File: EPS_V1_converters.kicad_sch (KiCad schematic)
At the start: 46 parts, among them U2 TPS62132RGTR, U3 TPS62133RGTR, U4 MP28167GQ-Z, U6 TPS61088RHLR

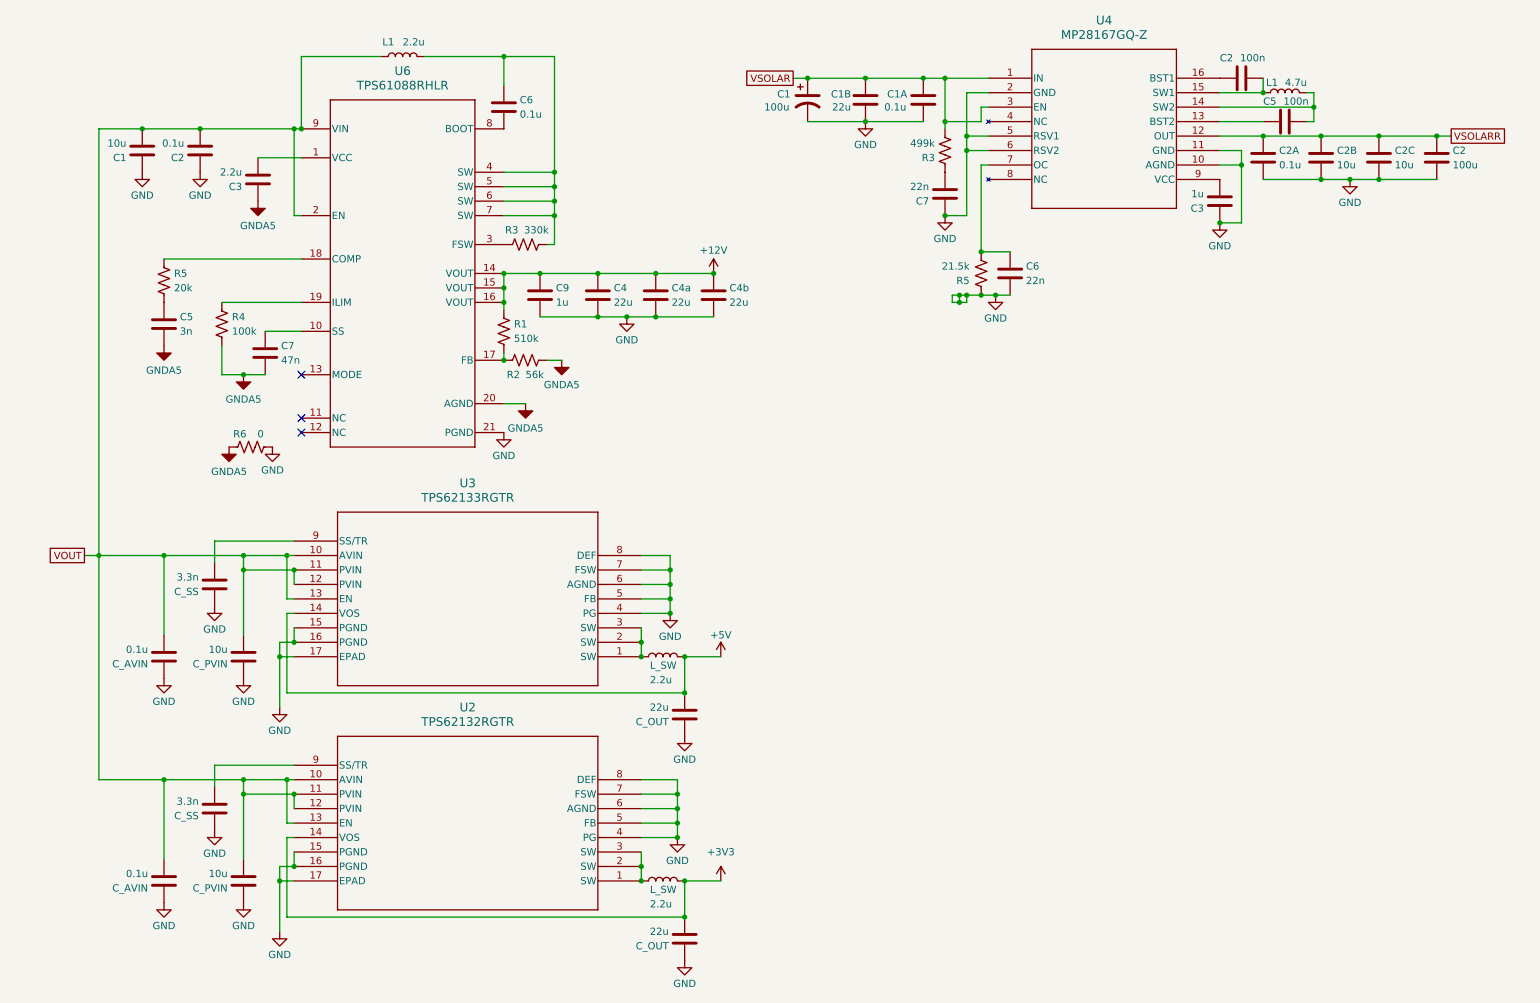
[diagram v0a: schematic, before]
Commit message: Clarify global net naming, other minor fixes
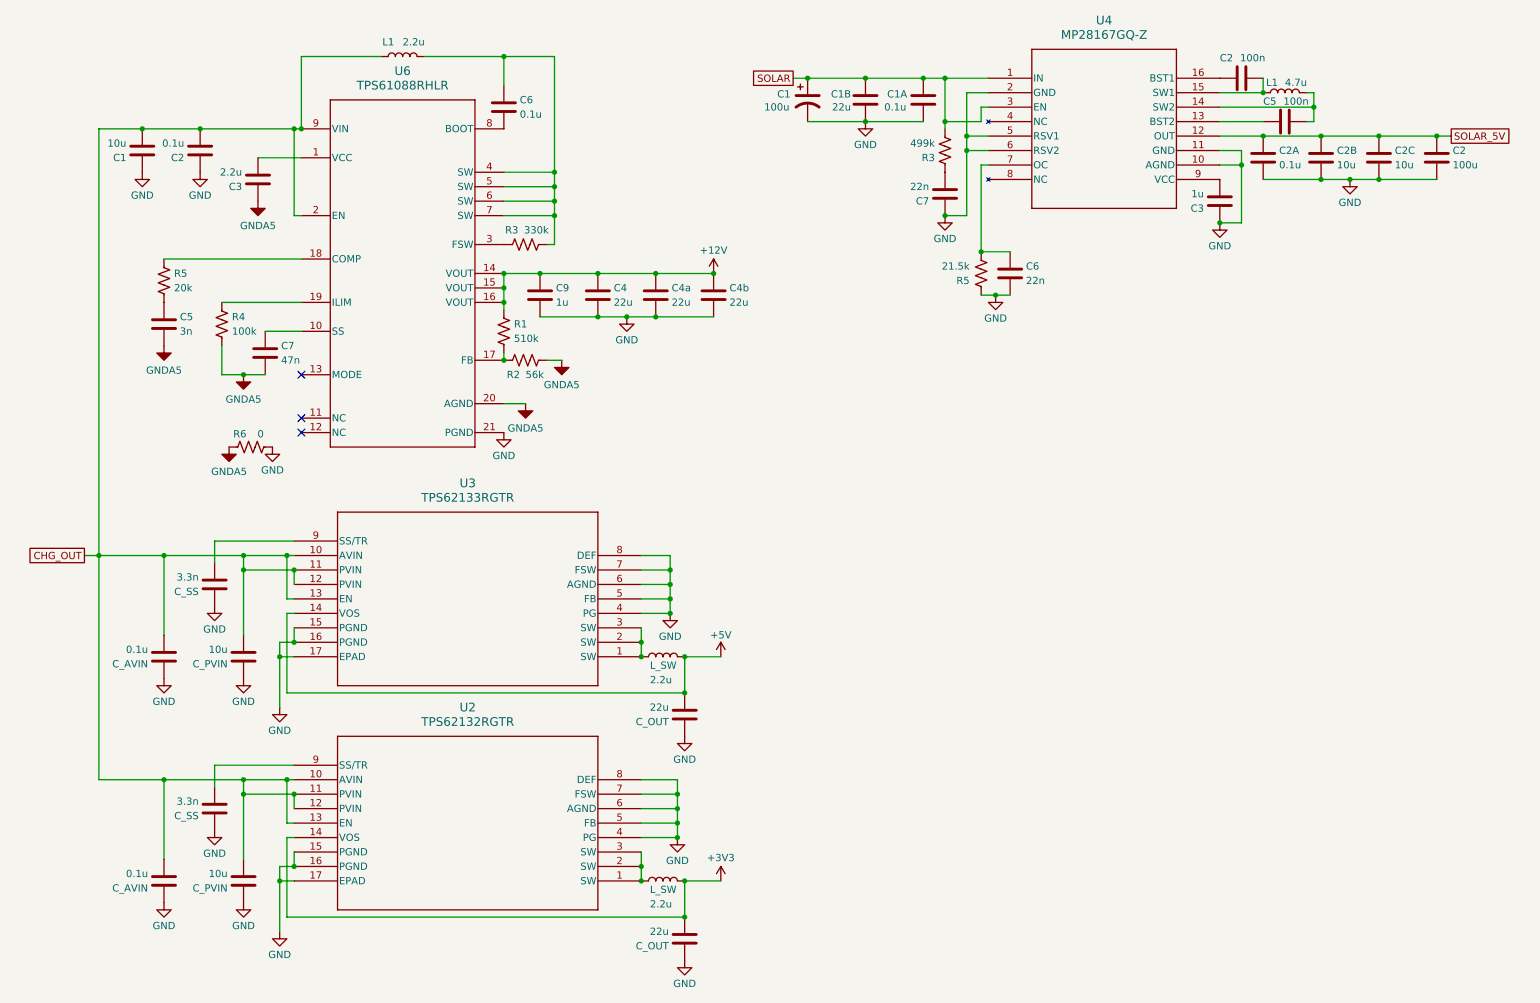
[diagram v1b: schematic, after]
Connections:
- net VOUT renamed CHG_OUT
- net VSOLAR renamed SOLAR
- net VSOLARR renamed SOLAR_5V
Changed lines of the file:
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@@
-	)
-	(junction
-		(at 186.69 68.58)
-		(diameter 0)
-		(color 0 0 0 0)
 	)
 	(junction
@@
 	)
 	(junction
-		(at 185.42 68.58)
-		(diameter 0)
-		(color 0 0 0 0)
-	)
-	(junction
 		(at 132.08 72.39)
 		(diameter 0)
@@
 	)
 	(junction
-		(at 189.23 68.58)
-		(diameter 0)
-		(color 0 0 0 0)
-	)
-	(junction
 		(at 114.3 49.53)
 		(diameter 0)
@@
 	(junction
 		(at 68.58 39.37)
-		(diameter 0)
-		(color 0 0 0 0)
-	)
-	(junction
-		(at 185.42 69.85)
 		(diameter 0)
 		(color 0 0 0 0)
@@
 	(wire
 		(pts
-			(xy 189.23 68.58) (xy 186.69 68.58)
-		)
-		(stroke
-			(width 0)
-			(type default)
-		)
-	)
-	(wire
-		(pts
 			(xy 114.3 59.69) (xy 113.03 59.69)
 		)
@@
 	(wire
 		(pts
-			(xy 186.69 68.58) (xy 186.69 69.85)
-		)
-		(stroke
-			(width 0)
-			(type default)
-		)
-	)
-	(wire
-		(pts
 			(xy 186.69 33.02) (xy 190.5 33.02)
 		)
@@
 	(wire
 		(pts
-			(xy 184.15 69.85) (xy 185.42 69.85)
-		)
-		(stroke
-			(width 0)
-			(type default)
-		)
-	)
-	(wire
-		(pts
 			(xy 190.5 35.56) (xy 189.23 35.56)
 		)
@@
 	(wire
 		(pts
-			(xy 185.42 68.58) (xy 185.42 69.85)
-		)
-		(stroke
-			(width 0)
-			(type default)
-		)
-	)
-	(wire
-		(pts
 			(xy 105.41 49.53) (xy 114.3 49.53)
 		)
@@
 	(wire
 		(pts
-			(xy 184.15 68.58) (xy 184.15 69.85)
-		)
-		(stroke
-			(width 0)
-			(type default)
-		)
-	)
-	(wire
-		(pts
 			(xy 105.41 46.99) (xy 114.3 46.99)
 		)
@@
 	(wire
 		(pts
-			(xy 185.42 68.58) (xy 184.15 68.58)
-		)
-		(stroke
-			(width 0)
-			(type default)
-		)
-	)
-	(wire
-		(pts
 			(xy 34.29 153.67) (xy 45.72 153.67)
 		)
@@
 	(wire
 		(pts
-			(xy 186.69 68.58) (xy 185.42 68.58)
-		)
-		(stroke
-			(width 0)
-			(type default)
-		)
-	)
-	(wire
-		(pts
 			(xy 186.69 43.18) (xy 190.5 43.18)
 		)
@@
 	(wire
 		(pts
-			(xy 185.42 69.85) (xy 186.69 69.85)
-		)
-		(stroke
-			(width 0)
-			(type default)
-		)
-	)
-	(wire
-		(pts
 			(xy 168.91 30.48) (xy 179.07 30.48)
 		)
@@
 		)
 	)
-	(global_label "VSOLAR"
+	(global_label "SOLAR"
 		(shape passive)
 		(at 156.21 30.48 180)
@@
 		)
 		(property "Intersheetrefs" "${INTERSHEET_REFS}"
-			(at 147.3208 30.48 0)
+			(at 148.4094 30.48 0)
 			(effects
 				(font
@@
 		)
 	)
-	(global_label "VSOLARR"
+	(global_label "SOLAR_5V"
 		(shape passive)
 		(at 271.78 40.64 0)
@@
 		)
 		(property "Intersheetrefs" "${INTERSHEET_REFS}"
-			(at 281.9392 40.64 0)
+			(at 282.8463 40.64 0)
 			(effects
 				(font
@@
 		)
 	)
-	(global_label "VOUT"
+	(global_label "CHG_OUT"
 		(shape passive)
 		(at 31.75 114.3 180)
@@
 		)
 		(property "Intersheetrefs" "${INTERSHEET_REFS}"
-			(at 25.1589 114.3 0)
+			(at 21.4094 114.3 0)
 			(effects
 				(font
@@
 		(on_board yes)
 		(dnp no)
-		(fields_autoplaced yes)
 		(property "Reference" "#PWR016"
 			(at 143.51 175.26 0)
@@
 		)
 		(property "Value" "+3V3"
-			(at 143.51 166.37 0)
-			(effects
-				(font
+			(at 143.51 167.386 0)
+			(effects
+				(font
